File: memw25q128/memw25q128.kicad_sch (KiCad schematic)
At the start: 15 parts, among them J1 STM32WORLD_BASE, U1 W25Q128JVS

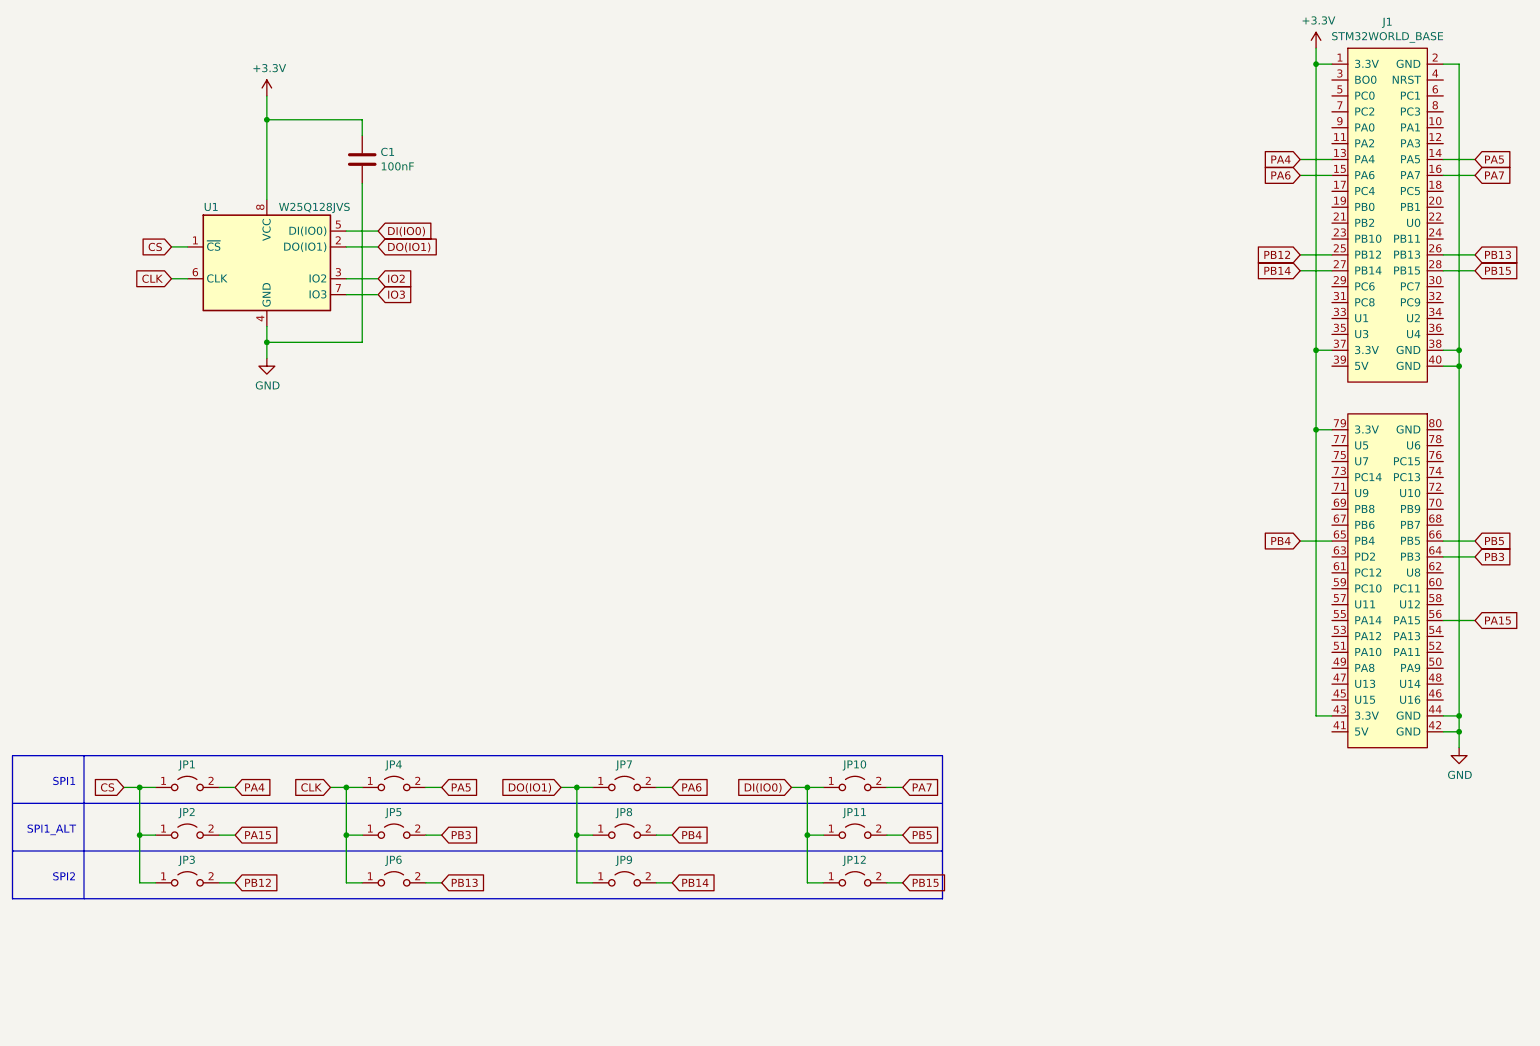
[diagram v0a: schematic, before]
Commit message: Hmmmm
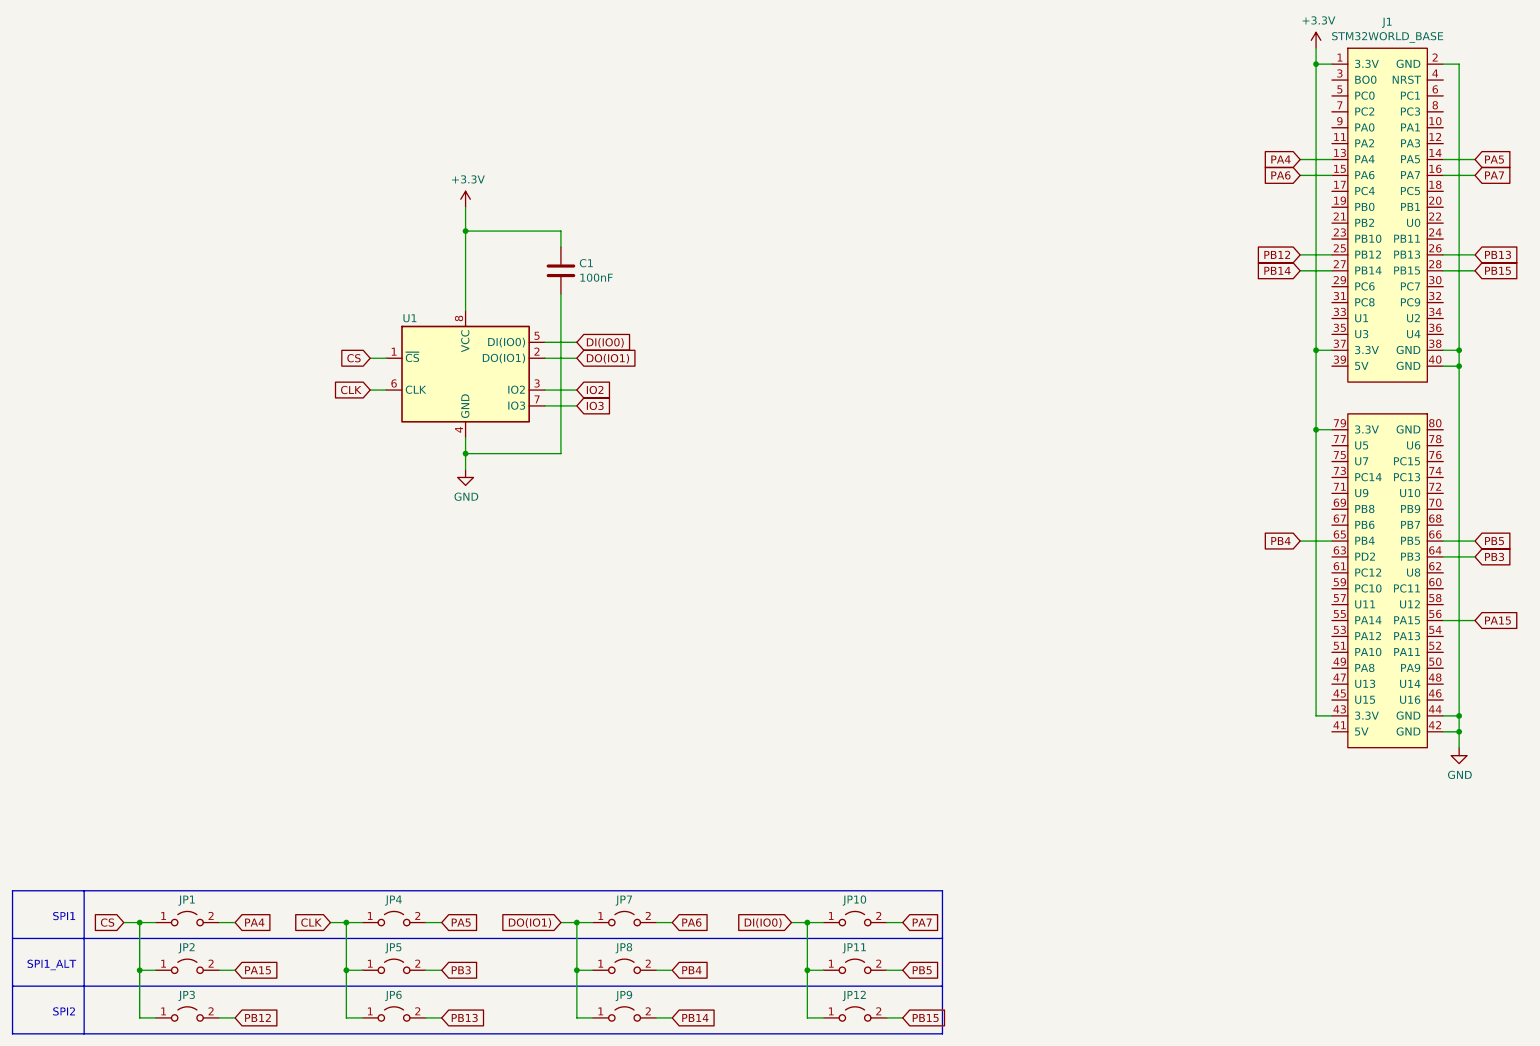
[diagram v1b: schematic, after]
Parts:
- U1: value W25Q128JVS -> (none); footprint Package_SO:SOIC-8_5.275x5.275mm_P1.27mm -> (none)
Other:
- company: (none) -> ${COMPANY}
- title: (none) -> ${TITLE}
- moved on the sheet: C1, JP1, JP10, JP11, JP12, JP2, JP3, JP4, JP5, JP6, JP7, JP8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
